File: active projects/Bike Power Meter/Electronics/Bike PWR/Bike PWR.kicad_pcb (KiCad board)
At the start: 4 copper layers, 55 x 55 mm, 26 parts, among them J1 Batt Holder, J3 Analyzer / Flasher, J4 Bridge, U1 LSM6DSLTR, U3 ScioSense PS09

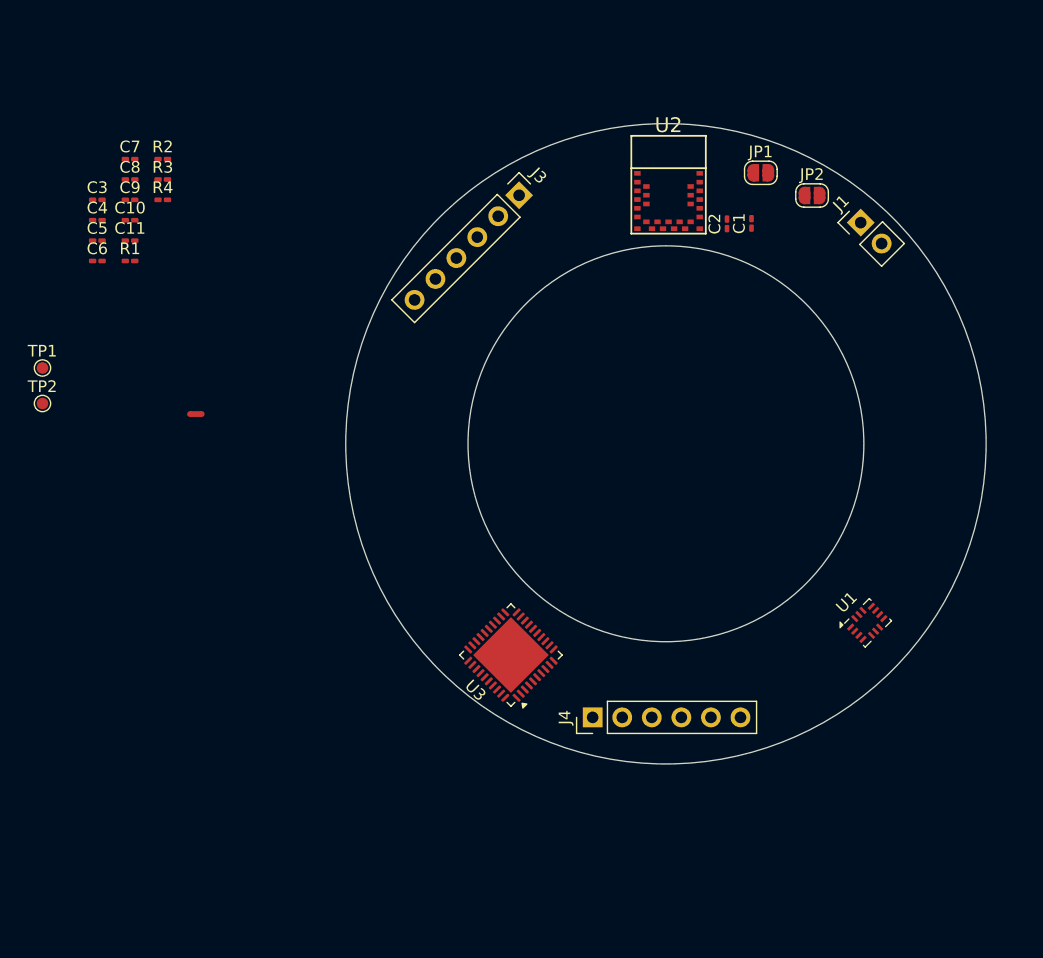
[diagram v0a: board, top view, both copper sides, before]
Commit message: Daily update: 2026-08-18 17:32:45
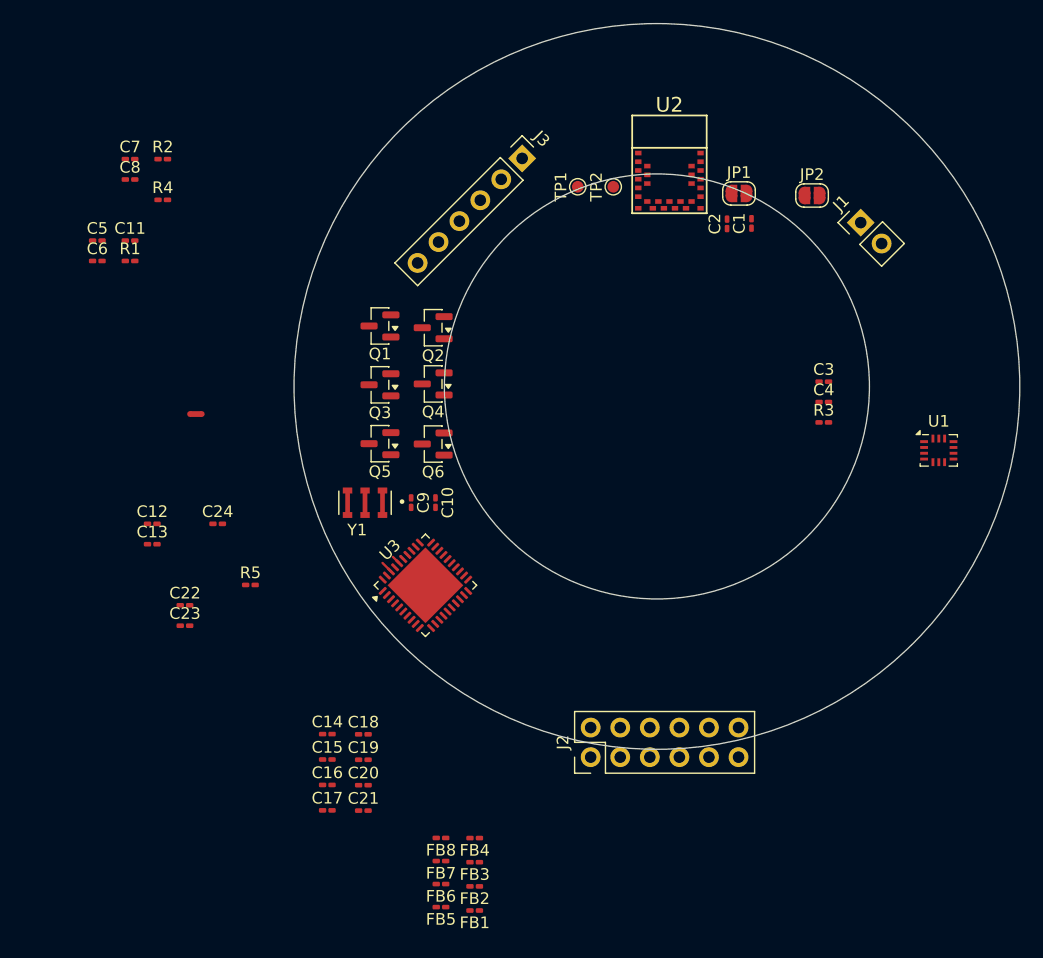
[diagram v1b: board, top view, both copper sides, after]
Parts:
- removed J4: Bridge, Connector_PinHeader_2.54mm:PinHeader_1x06_P2.54mm_Vertical
- added C12: 100uF, Capacitor_SMD:C_0201_0603Metric_Pad0.64x0.40mm_HandSolder, F.Cu at (126.7, 111.8)
- added C13: 100nF, Capacitor_SMD:C_0201_0603Metric_Pad0.64x0.40mm_HandSolder, F.Cu at (126.7, 113.5)
- added C14: 470pF, Capacitor_SMD:C_0201_0603Metric_Pad0.64x0.40mm_HandSolder, F.Cu at (141.7, 129.9)
- added C15: 470pF, Capacitor_SMD:C_0201_0603Metric_Pad0.64x0.40mm_HandSolder, F.Cu at (141.7, 132.0)
- added C16: 470pF, Capacitor_SMD:C_0201_0603Metric_Pad0.64x0.40mm_HandSolder, F.Cu at (141.7, 134.2)
- added C17: 470pF, Capacitor_SMD:C_0201_0603Metric_Pad0.64x0.40mm_HandSolder, F.Cu at (141.7, 136.4)
- added C18: 470pF, Capacitor_SMD:C_0201_0603Metric_Pad0.64x0.40mm_HandSolder, F.Cu at (144.8, 129.9)
- added C19: 470pF, Capacitor_SMD:C_0201_0603Metric_Pad0.64x0.40mm_HandSolder, F.Cu at (144.8, 132.1)
- added C20: 470pF, Capacitor_SMD:C_0201_0603Metric_Pad0.64x0.40mm_HandSolder, F.Cu at (144.8, 134.2)
- added C21: 470pF, Capacitor_SMD:C_0201_0603Metric_Pad0.64x0.40mm_HandSolder, F.Cu at (144.8, 136.4)
- added C22: 100pF, Capacitor_SMD:C_0201_0603Metric_Pad0.64x0.40mm_HandSolder, F.Cu at (129.5, 118.8)
- added C23: 3.3nF, Capacitor_SMD:C_0201_0603Metric_Pad0.64x0.40mm_HandSolder, F.Cu at (129.5, 120.5)
- added C24: 33uF, Capacitor_SMD:C_0201_0603Metric_Pad0.64x0.40mm_HandSolder, F.Cu at (132.3, 111.8)
- added FB1: 220/0.05, Inductor_SMD:L_0201_0603Metric_Pad0.64x0.40mm_HandSolder, F.Cu at (154.4, 145.0)
- added FB2: 220/0.05, Inductor_SMD:L_0201_0603Metric_Pad0.64x0.40mm_HandSolder, F.Cu at (154.4, 142.9)
- added FB3: 220/0.05, Inductor_SMD:L_0201_0603Metric_Pad0.64x0.40mm_HandSolder, F.Cu at (154.4, 140.9)
- added FB4: 220/0.05, Inductor_SMD:L_0201_0603Metric_Pad0.64x0.40mm_HandSolder, F.Cu at (154.4, 138.8)
- added FB5: 220/0.05, Inductor_SMD:L_0201_0603Metric_Pad0.64x0.40mm_HandSolder, F.Cu at (151.5, 144.7)
- added FB6: 220/0.05, Inductor_SMD:L_0201_0603Metric_Pad0.64x0.40mm_HandSolder, F.Cu at (151.5, 142.7)
- added FB7: 220/0.05, Inductor_SMD:L_0201_0603Metric_Pad0.64x0.40mm_HandSolder, F.Cu at (151.5, 140.8)
- added FB8: 220/0.05, Inductor_SMD:L_0201_0603Metric_Pad0.64x0.40mm_HandSolder, F.Cu at (151.5, 138.8)
- added J2: Bridge, Connector_PinHeader_2.54mm:PinHeader_2x06_P2.54mm_Vertical, F.Cu at (164.3, 131.8)
- added Q1: BC857, Package_TO_SOT_SMD:SOT-23, F.Cu at (146.2, 94.8)
- added Q2: BC857, Package_TO_SOT_SMD:SOT-23, F.Cu at (150.8, 95.0)
- added Q3: BC857, Package_TO_SOT_SMD:SOT-23, F.Cu at (146.2, 99.9)
- added Q4: BC857, Package_TO_SOT_SMD:SOT-23, F.Cu at (150.8, 99.8)
- added Q5: BC857, Package_TO_SOT_SMD:SOT-23, F.Cu at (146.2, 104.9)
- added Q6: BC857, Package_TO_SOT_SMD:SOT-23, F.Cu at (150.8, 104.9)
- added R5: 3.3k, Resistor_SMD:R_0201_0603Metric_Pad0.64x0.40mm_HandSolder, F.Cu at (135.1, 117.0)
- added Y1: Resonator, bike:OSC_CSTCR4M00G53-R0, F.Cu at (144.9, 110.0)
- U1: value LSM6DSLTR -> BMI160
- moved C3 64.3 mm to (184.3, 99.6)
- moved C4 64.3 mm to (184.3, 101.3)
- moved R3 60.5 mm to (184.3, 103.1)
- moved TP2 52.4 mm to (166.2, 82.8), turned to 90 degrees
- moved TP1 48.5 mm to (163.2, 82.8), turned to 90 degrees
- moved C10 35.7 mm to (151.0, 110.0), turned to -90 degrees
- moved C9 35.5 mm to (148.9, 110.0), turned to -90 degrees
- moved U1 16.0 mm to (194.2, 105.5), turned to 0 degrees
- moved U3 9.48 mm to (150.1, 117.1), turned to 45 degrees
- moved J3 3.18 mm to (158.4, 80.4)
- moved JP1 2.58 mm to (177.1, 83.4)
- moved U2 1.75 mm to (171.1, 82.3)
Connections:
- J3 pad 2: SWFIO -> SWDIO
- U1 pad 10: (no net) -> unconnected-(U1-OCSB-Pad10)
- U1 pad 11: (no net) -> unconnected-(U1-OSDO-Pad11)
- U3 pad 12: MULT_IO7_CREF -> unconnected-(U3-MULT_IO7_CREF-Pad12)
- U3 pad 13: SG_B -> SG_B1
- U3 pad 14: SG_B -> SG_B2
- U3 pad 15: SG_A -> SG_A1
- U3 pad 16: SG_A -> SG_A2
- U3 pad 18: VCC_LOAD -> VDD
- U3 pad 2: unconnected-(U3-MULT_IO3_C1-Pad2) -> TDC_INTN
- U3 pad 20: LOAD_LINE -> LOAD
- U3 pad 23: SG_C -> SG_C2
- U3 pad 24: SG_C -> SG_C1
- U3 pad 25: SG_D -> SG_D2
- U3 pad 26: SG_D -> SG_D1
- U3 pad 27: TDC_INTN -> unconnected-(U3-MULT_IO5_C3-Pad27)
- U3 pad 34: unconnected-(U3-RCOMP-Pad34) -> RCOMP
- U3 pad 35: unconnected-(U3-CCOMP-Pad35) -> CCOMP
- U3 pad 36: unconnected-(U3-UCOMP-Pad36) -> UCOMP
- U3 pad 38: unconnected-(U3-XT1-Pad38) -> Net-(U3-XT1)
- U3 pad 39: unconnected-(U3-XT2-Pad39) -> Net-(U3-XT2)
- U3 pad 8: unconnected-(U3-EE_DATA-Pad8) -> Net-(U3-EE_DATA)
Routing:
- net Net-(U3-XT1): track 0.00 -> 1.03 mm
- net UCOMP: track 0.00 -> 0.76 mm
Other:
- board size 55 x 55 mm -> 62.3 x 62.3 mm
